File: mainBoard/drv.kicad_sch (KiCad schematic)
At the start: 9 parts, among them J8 Conn_01x02, M1 Conn_01x01, M2 Conn_01x01, U3 DRV8251ADDAR

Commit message: Zvetšení test pointů
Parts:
- TP1, TP2: footprint Connector_Pin:Pin_D0.7mm_L6.5mm_W1.8mm_FlatFork -> Connector_Pin:Pin_D1.0mm_L10.0mm
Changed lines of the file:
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@@
       (effects (font (size 1.27 1.27)) (justify left))
     )
-    (property "Footprint" "Connector_Pin:Pin_D0.7mm_L6.5mm_W1.8mm_FlatFork" (at 132.08 99.06 0)
+    (property "Footprint" "Connector_Pin:Pin_D1.0mm_L10.0mm" (at 132.08 99.06 0)
       (effects (font (size 1.27 1.27)) hide)
     )
@@
       (effects (font (size 1.27 1.27)) (justify left))
     )
-    (property "Footprint" "Connector_Pin:Pin_D0.7mm_L6.5mm_W1.8mm_FlatFork" (at 139.7 99.06 0)
+    (property "Footprint" "Connector_Pin:Pin_D1.0mm_L10.0mm" (at 139.7 99.06 0)
       (effects (font (size 1.27 1.27)) hide)
     )

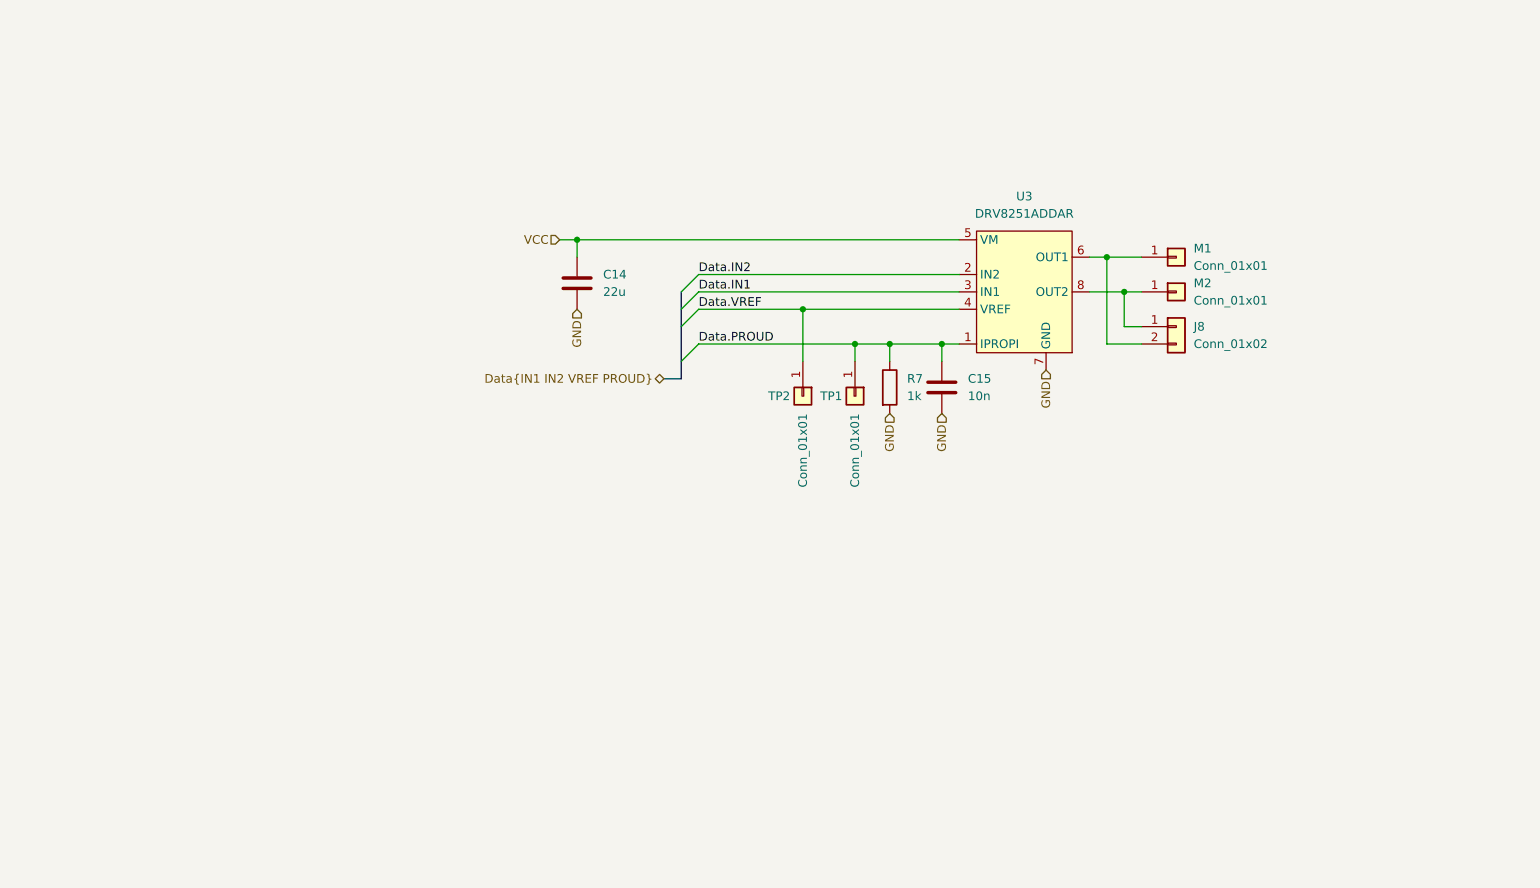
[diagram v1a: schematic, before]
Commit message: Moc kondíků
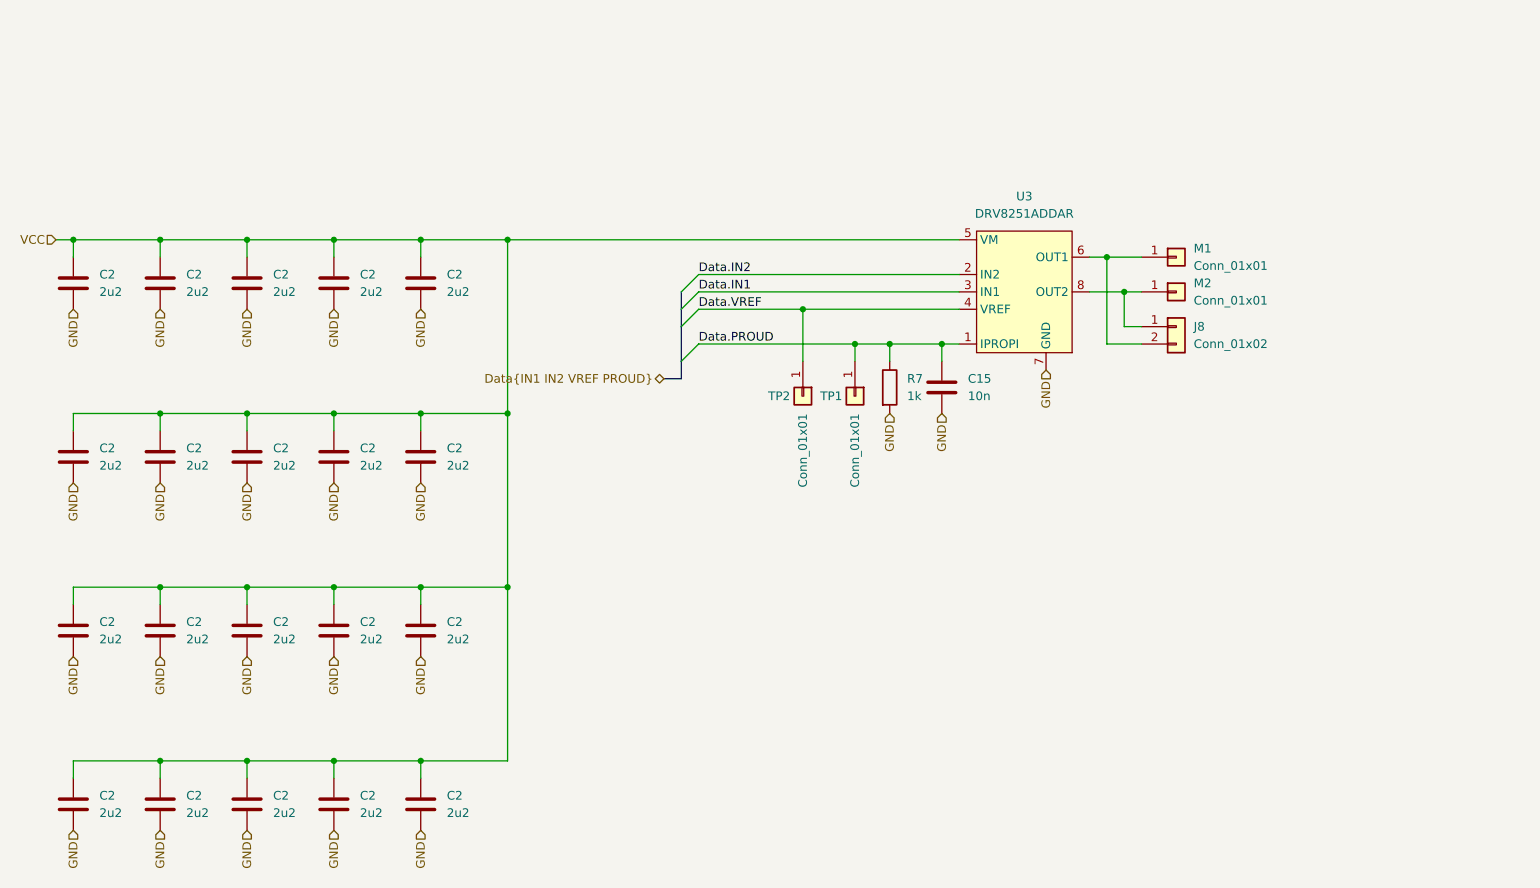
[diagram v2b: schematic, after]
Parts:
- removed C14: 22u, Capacitor_SMD:C_2220_5650Metric, symbol Device:C
- added C2 (x20): 2u2, Capacitor_SMD:C_0805_2012Metric, symbol Device:C
- J8: footprint Connector_Phoenix_MC:PhoenixContact_MCV_1,5_2-G-3.81_1x02_P3.81mm_Vertical -> Connector_JST:JST_XH_B2B-XH-AM_1x02_P2.50mm_Vertical
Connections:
- net GND: now also C2.2, C2.2, C2.2, C2.2, C2.2, C2.2, C2.2, C2.2, C2.2, C2.2, C2.2, C2.2, C2.2, C2.2, C2.2, C2.2, C2.2, C2.2, C2.2, C2.2
- net VCC: now also C2.1, C2.1, C2.1, C2.1, C2.1, C2.1, C2.1, C2.1, C2.1, C2.1, C2.1, C2.1, C2.1, C2.1, C2.1, C2.1, C2.1, C2.1, C2.1, C2.1

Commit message: GNDDETECT
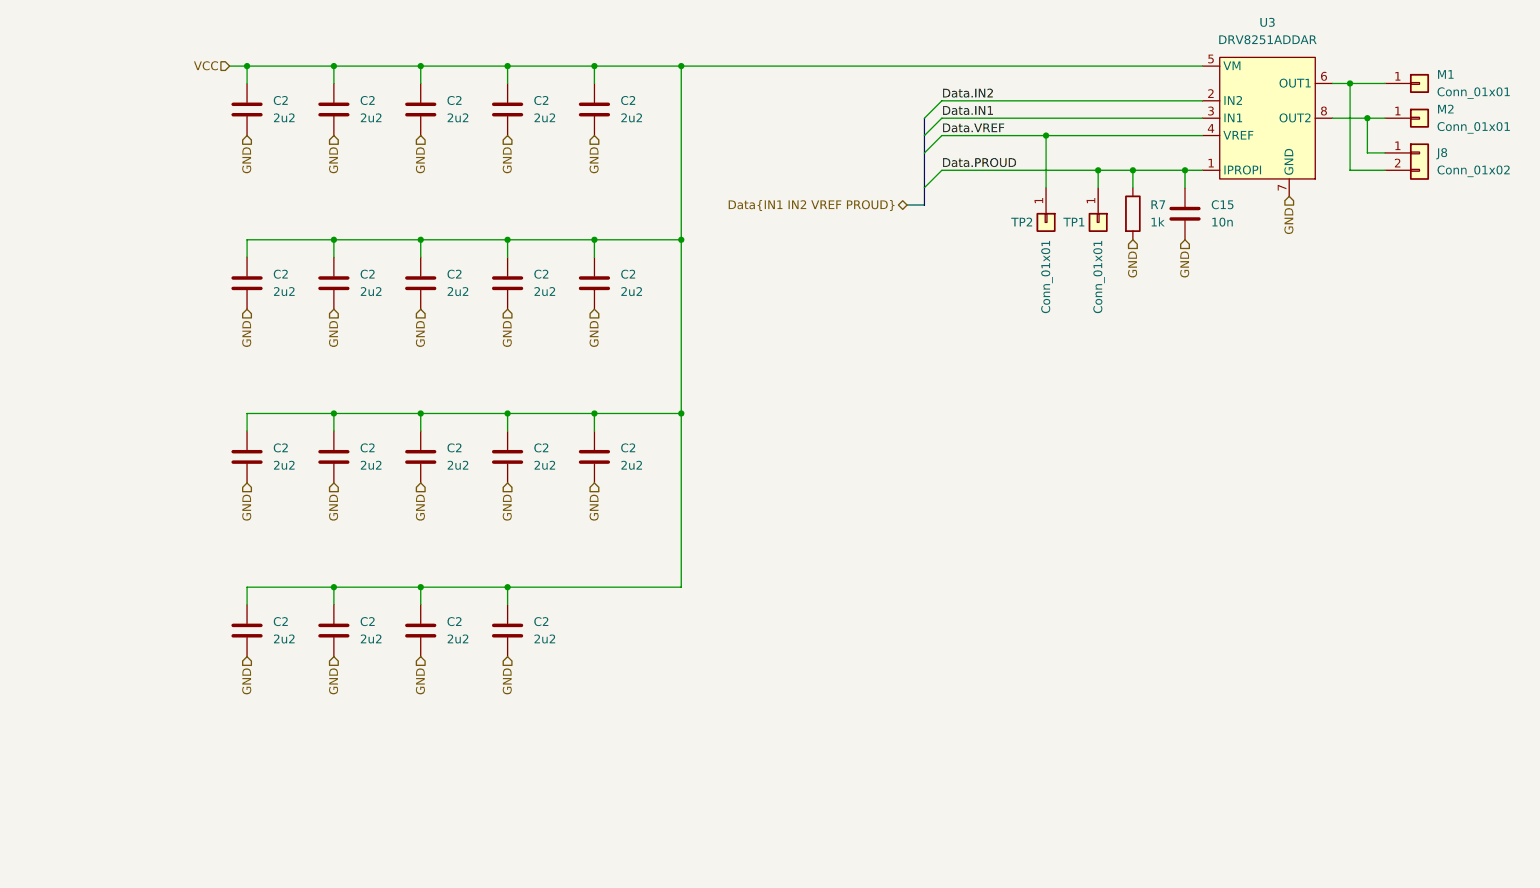
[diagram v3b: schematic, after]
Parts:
- removed C2: 2u2, Capacitor_SMD:C_0805_2012Metric, symbol Device:C
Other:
- moved on the sheet: C15, C2, J8, M1, M2, R7, TP1, TP2, U3

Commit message: 16x20
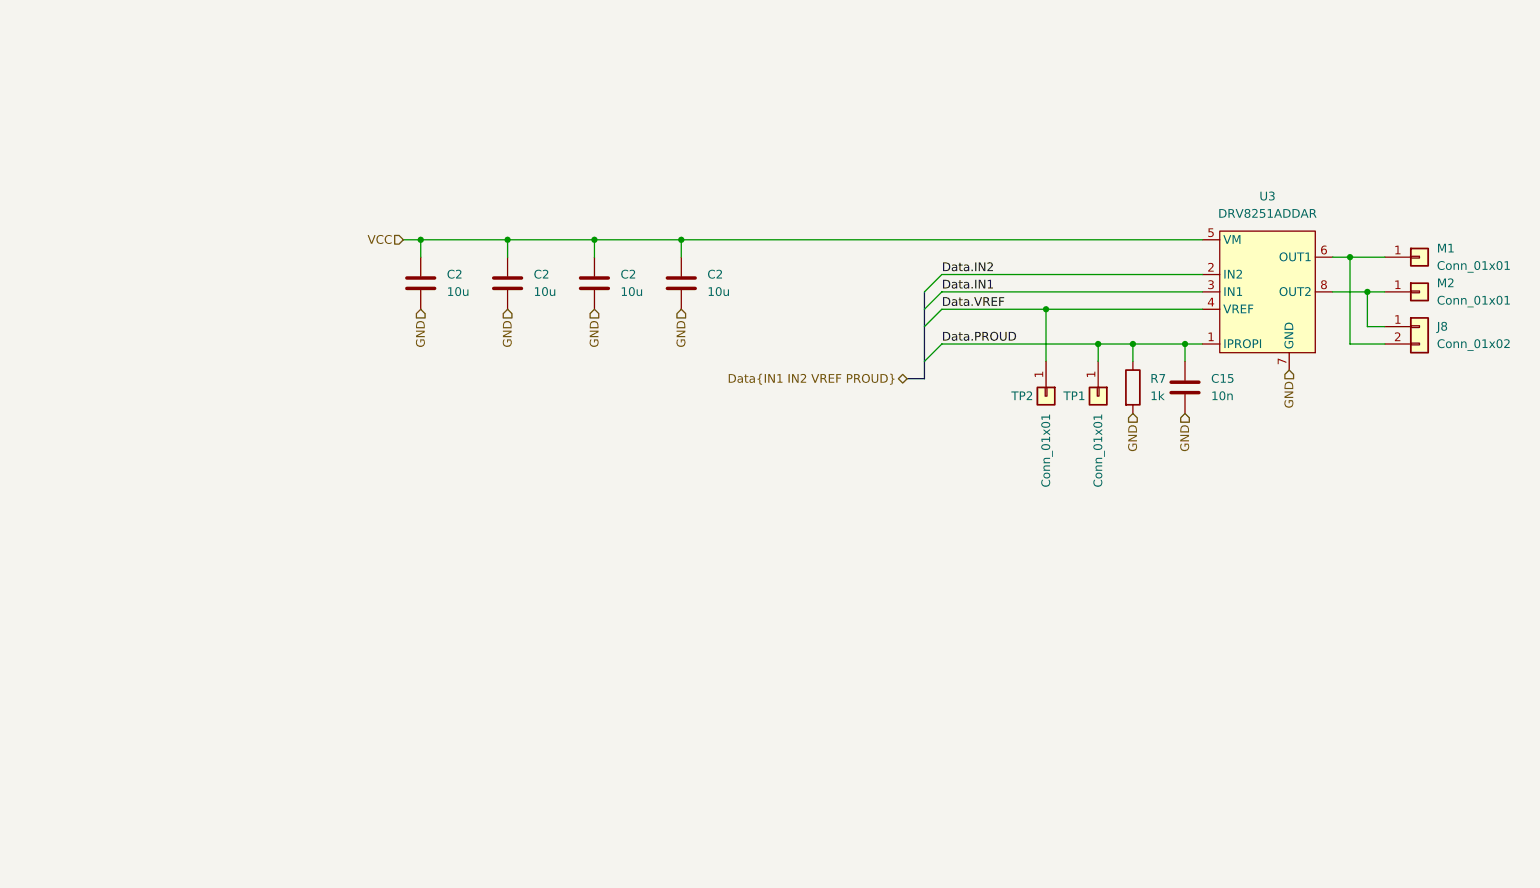
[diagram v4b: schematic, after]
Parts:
- removed C2 (x19): 2u2, Capacitor_SMD:C_0805_2012Metric, symbol Device:C
- added C2 (x4): 10u, Capacitor_SMD:C_0805_2012Metric, symbol Device:C
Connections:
- net GND: now also C2.2, C2.2, C2.2, C2.2
- net VCC: now also C2.1, C2.1, C2.1, C2.1
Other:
- moved on the sheet: C15, J8, M1, M2, R7, TP1, TP2, U3

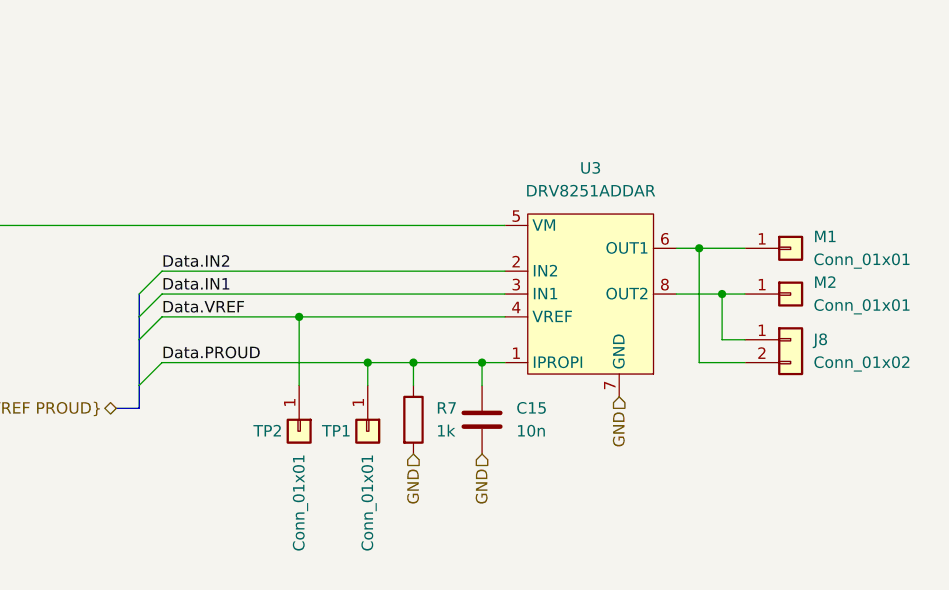
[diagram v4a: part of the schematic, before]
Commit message: drobeček
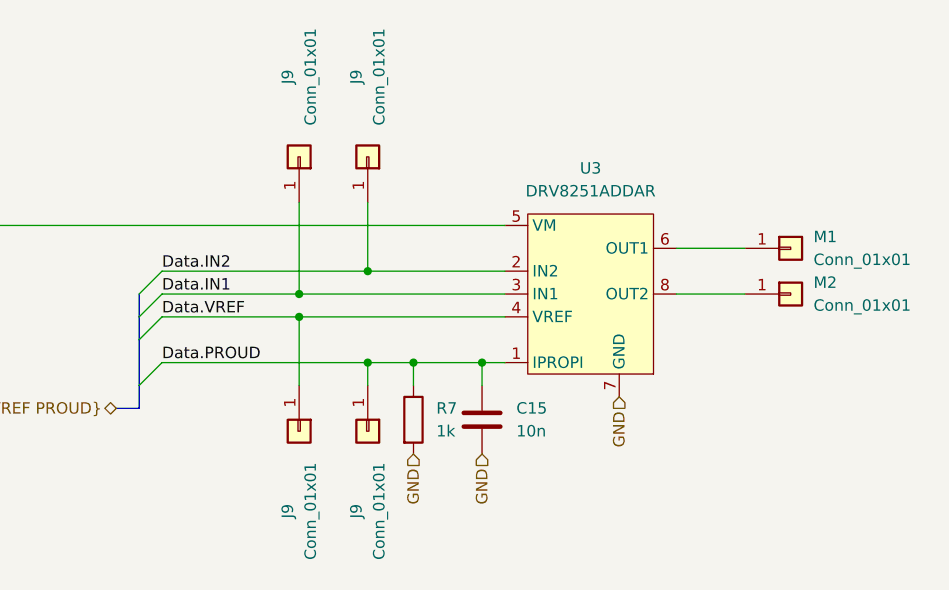
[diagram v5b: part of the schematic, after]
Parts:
- removed J8: Conn_01x02, Connector_JST:JST_XH_B2B-XH-AM_1x02_P2.50mm_Vertical, symbol Connector_Generic:Conn_01x02
- removed TP1, TP2: Conn_01x01, Connector_Pin:Pin_D1.0mm_L10.0mm, symbol Connector_Generic:Conn_01x01
- added J9 (x4): Conn_01x01, RKL-Connectors:YZ157015035P-01-contact_pad, symbol Connector_Generic:Conn_01x01
- C15: footprint Capacitor_SMD:C_0402_1005Metric -> Capacitor_SMD:C_0201_0603Metric; LCSC C15195 -> C285010
- C2: footprint Capacitor_SMD:C_0805_2012Metric -> Capacitor_SMD:C_0603_1608Metric; LCSC C440198 -> C194427; note 50V, X5R -> 35V, X5R
- M1, M2: footprint Connector_Pin:Pin_D1.0mm_L10.0mm -> RKL-Connectors:YZ157015035P-01-contact_pad
- R7: footprint Capacitor_SMD:C_0402_1005Metric -> Capacitor_SMD:C_0201_0603Metric; LCSC C852624 -> C138165
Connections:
- net Data.IN1: now also J9.1 (Pin_1)
- net Data.IN2: now also J9.1 (Pin_1)
- net Data.PROUD: now also J9.1 (Pin_1)
- net Data.VREF: now also J9.1 (Pin_1)
